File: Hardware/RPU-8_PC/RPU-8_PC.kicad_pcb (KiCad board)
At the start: 4 copper layers, 139.7 x 55.9 mm, 11 parts, among them J1 ADDR_BUS, J2 DATA_BUS, J3 Conn_01x03_Female, J4 CTRL_BUS, J5 INST_REG, U1 74HC161, U2 74HC245, U3 74HC161, U4 74HC161, U5 74HC245, U6 74HC161

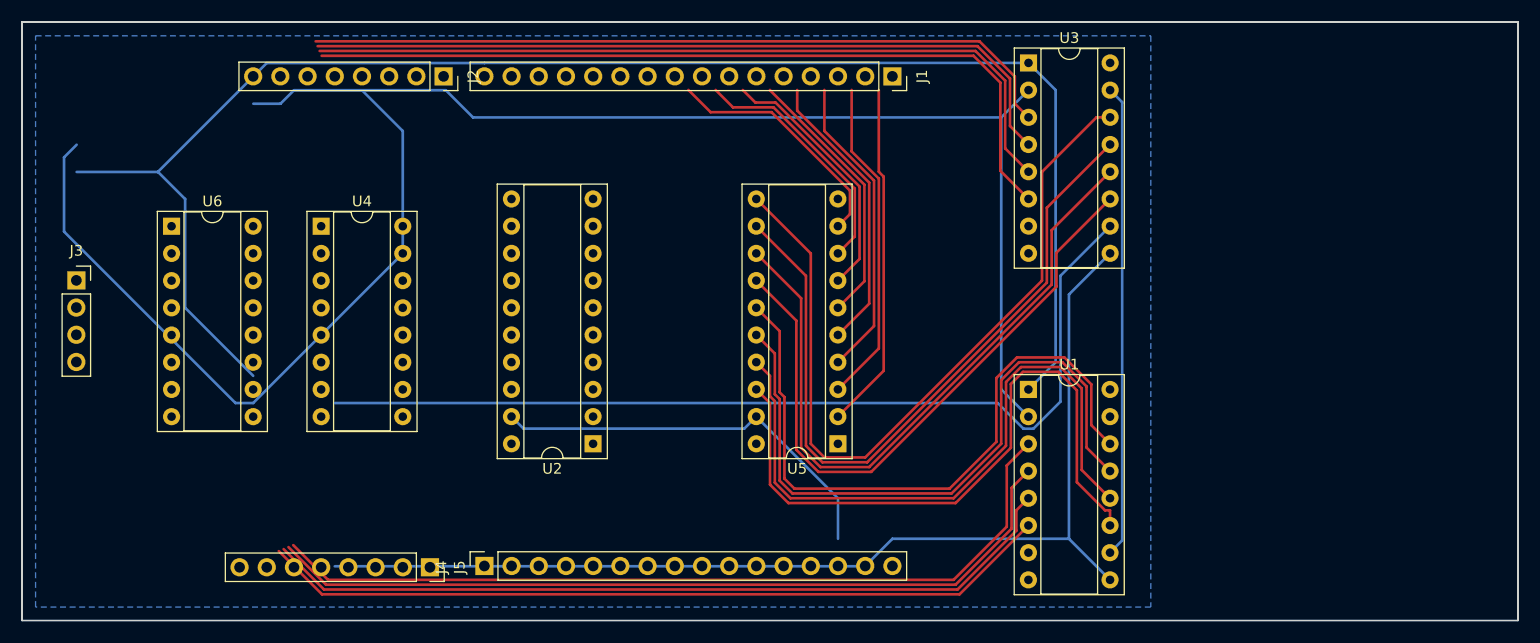
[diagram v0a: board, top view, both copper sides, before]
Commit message: add .readthedocs.yaml
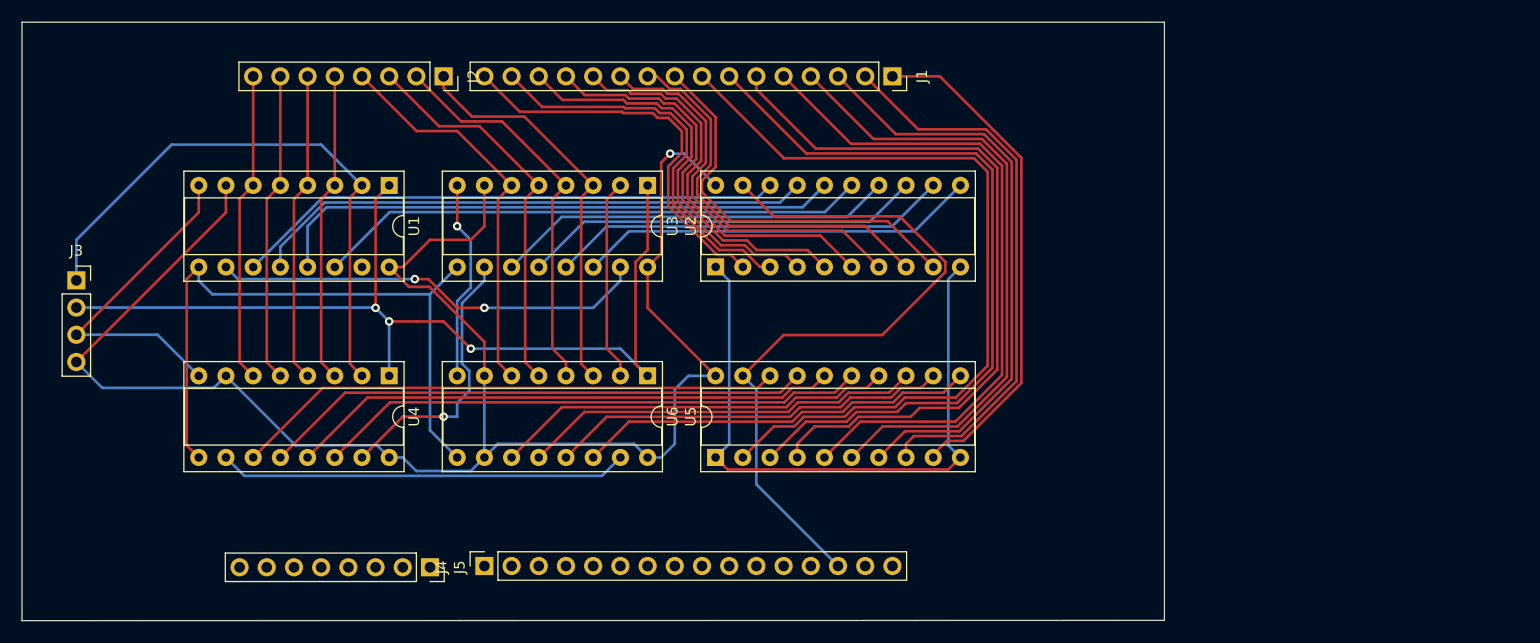
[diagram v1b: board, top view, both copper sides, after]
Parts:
- moved U1 62.7 mm to (102.9, 83.8), turned to -90 degrees
- moved U6 46.6 mm to (127.0, 101.6), turned to -90 degrees
- moved U3 37.4 mm to (127.0, 83.8), turned to -90 degrees
- moved U2 20.1 mm to (133.4, 91.4), turned to 90 degrees
- moved U4 15.3 mm to (102.9, 101.6), turned to -90 degrees
- moved U5 11.5 mm to (133.3, 109.2), turned to 90 degrees
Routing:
- net +5V: track 0.00 -> 161.4 mm, vias 0 -> 1
- net GND: track 0.00 -> 111.9 mm, vias 0 -> 1
- net CLK: track 173.5 -> 73.3 mm
- net Net-(U3-Pad10): track 88.1 -> 26.0 mm, vias 0 -> 1
- net RST: track 148.4 -> 91.7 mm, vias 0 -> 3
- net Net-(U4-Pad12): track 0.00 -> 51.4 mm
- net Net-(U4-Pad14): track 0.00 -> 51.4 mm
- net Net-(U4-Pad13): track 0.00 -> 51.4 mm
- net Net-(U4-Pad11): track 0.00 -> 51.4 mm
- net D4: track 78.6 -> 29.0 mm
- net D5: track 77.2 -> 29.0 mm
- net D6: track 75.8 -> 29.0 mm
- net D7: track 74.3 -> 29.0 mm
- net A7: track 32.5 -> 74.9 mm
- net ~{CIL}: track 103.3 -> 62.0 mm
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- removed copper zone on In2.Cu, net +5V
- removed copper zone on B.Cu, net GND
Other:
- board size 139.7 x 55.9 mm -> 106.7 x 55.9 mm
- copper layers 4 -> 2
